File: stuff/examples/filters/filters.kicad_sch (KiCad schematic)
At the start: 3 parts, among them U1 MAX7375AXR805

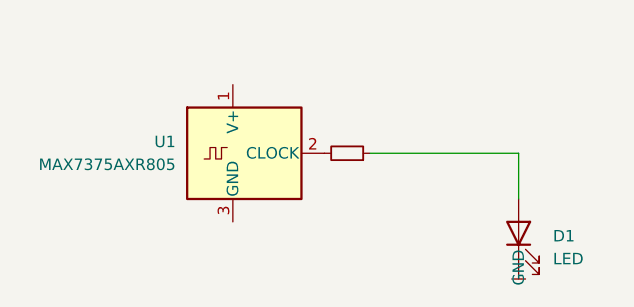
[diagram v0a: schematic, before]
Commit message: Transistor filter (uncompleted)
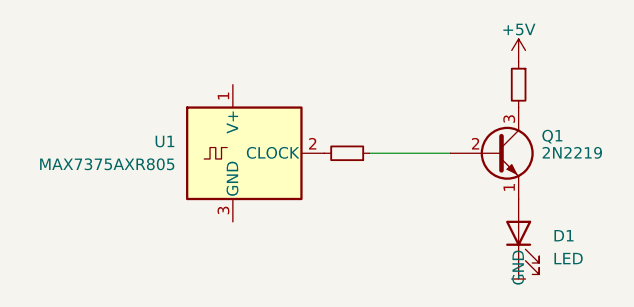
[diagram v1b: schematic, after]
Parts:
- added Q1: 2N2219, Package_TO_SOT_THT:TO-39-3, symbol Transistor_BJT:2N2219
- added R1: 100R, KIM-1_Library:R_Axial_DIN0309_100R_L6.3mm_D2.5mm_P12.70mm_Horizontal, symbol Device:R_Small
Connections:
- net at R6.1: now also Q1.2 (B); no longer D1.2 (A)
- new net: Q1.3 (C), R1.2
- new net: D1.2 (A), Q1.1 (E)
- new net +5V: R1.1
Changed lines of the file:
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@@
 (kicad_sch (version 20230121) (generator eeschema)
   (paper "A2")
-  (wire (pts (xy 334.01 67.31) (xy 334.01 62.23))
-    (stroke (width 0) (type default))
-  )
-  (wire (pts (xy 334.01 62.23) (xy 317.5 62.23))
+  (wire (pts (xy 326.39 62.23) (xy 317.5 62.23))
     (stroke (width 0) (type default))
   )
@@
         (path "/12882ae0-ee92-4cfd-99ea-b49ca74b2a9a"
           (reference "R6") (unit 1)
+        )
+      )
+    )
+  )
+  (symbol (lib_id "Device:R_Small") (at 334.01 54.61 0) (mirror y) (unit 1)
+    (in_bom yes) (on_board yes) (dnp no)
+    (property "Reference" "R1" (at 328.93 55.88 0)
+      (effects (font (size 1.27 1.27)) (justify right) hide)
+    )
+    (property "Value" "100R" (at 327.66 53.34 0)
+      (effects (font (size 1.27 1.27)) (justify right) hide)
+    )
+    (property "Footprint" "KIM-1_Library:R_Axial_DIN0309_100R_L6.3mm_D2.5mm_P12.70mm_Horizontal" (at 334.01 54.61 0)
+      (effects (font (size 1.27 1.27)) hide)
+    )
+    (property "Datasheet" "~" (at 334.01 54.61 0)
+      (effects (font (size 1.27 1.27)) hide)
+    )
+    (pin "1")
+    (pin "2")
+    (instances
+      (project "filters"
+        (path "/12882ae0-ee92-4cfd-99ea-b49ca74b2a9a"
+          (reference "R1") (unit 1)
         )
       )
@@
         )
       )
+    )
+  )
+  (symbol (lib_id "power:+5V") (at 334.01 52.07 0) (unit 1)
+    (in_bom yes) (on_board yes) (dnp no)
+    (property "Reference" "#PWR01" (at 334.01 55.88 0)
+      (effects (font (size 1.27 1.27)) hide)
+    )
+    (property "Value" "+5V" (at 334.01 48.514 0)
+      (effects (font (size 1.27 1.27)))
+    )
+    (property "Footprint" "" (at 334.01 52.07 0)
+      (effects (font (size 1.27 1.27)) hide)
+    )
+    (property "Datasheet" "" (at 334.01 52.07 0)
+      (effects (font (size 1.27 1.27)) hide)
+    )
+    (pin "1")
+    (instances
+      (project "filters"
+        (path "/12882ae0-ee92-4cfd-99ea-b49ca74b2a9a"
+          (reference "#PWR01") (unit 1)
+        )
+      )
+    )
+  )
+  (symbol (lib_id "Transistor_BJT:2N2219") (at 331.47 62.23 0) (unit 1)
+    (in_bom yes) (on_board yes) (dnp no)
+    (property "Reference" "Q1" (at 336.55 60.325 0)
+      (effects (font (size 1.27 1.27)) (justify left))
+    )
+    (property "Value" "2N2219" (at 336.55 62.23 0)
+      (effects (font (size 1.27 1.27)) (justify left))
+    )
+    (property "Footprint" "Package_TO_SOT_THT:TO-39-3" (at 336.55 64.135 0)
+      (effects (font (size 1.27 1.27) italic) (justify left) hide)
+    )
+    (property "Datasheet" "http://www.onsemi.com/pub_link/Collateral/2N2219-D.PDF" (at 331.47 62.23 0)
+      (effects (font (size 1.27 1.27)) (justify left) hide)
+    )
+    (pin "1")
+    (pin "3")
+    (pin "2")
+    (instances
+      (project "filters"
+        (path "/12882ae0-ee92-4cfd-99ea-b49ca74b2a9a"
+          (reference "Q1") (unit 1)
+        )
+      )
